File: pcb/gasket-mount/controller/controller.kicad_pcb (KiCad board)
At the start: 2 copper layers, 31.3 x 24.9 mm, 34 parts, among them J1 USB_C_Receptacle_USB2.0_16P, U1 USBLC6-2SC6, U3 W25Q128JVP, U4 RP2040, U5 AP2112K-3.3, X1 ABM8-272-T3

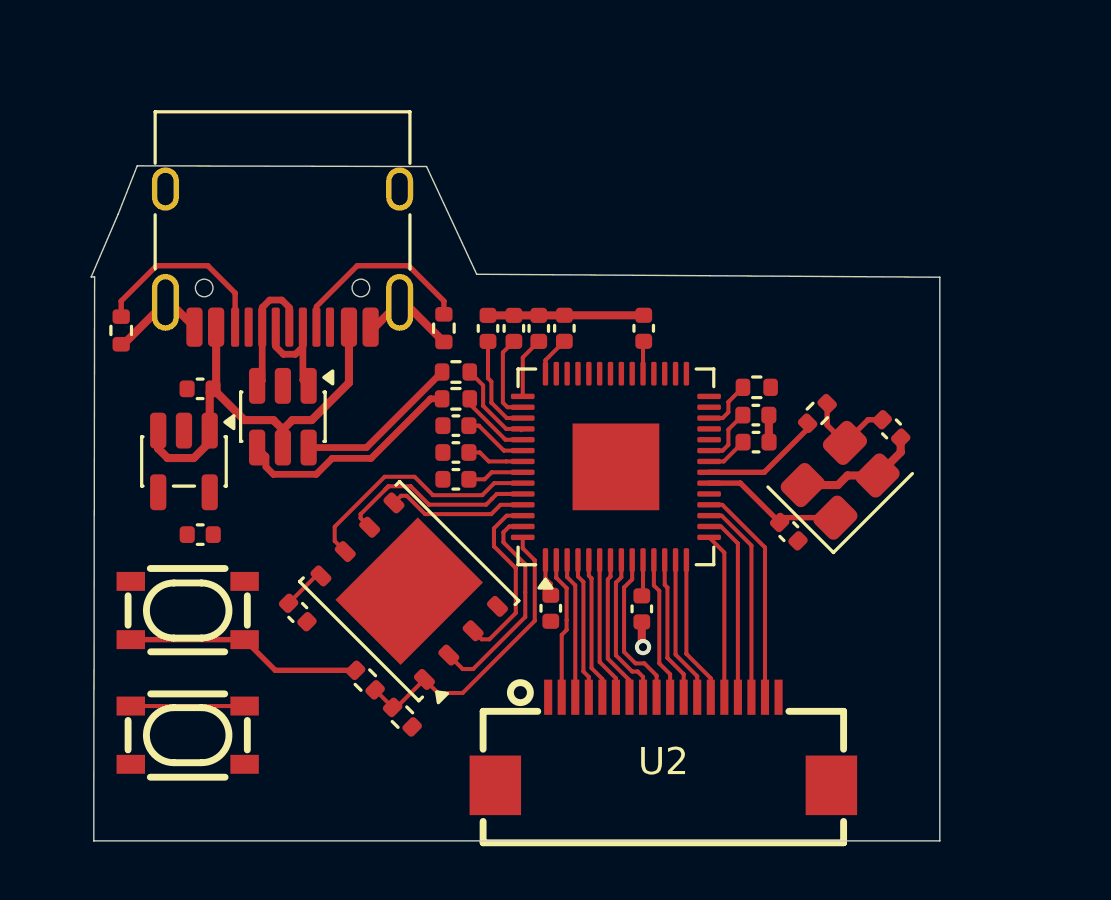
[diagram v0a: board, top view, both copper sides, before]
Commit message: Last commit before changing Flash memory
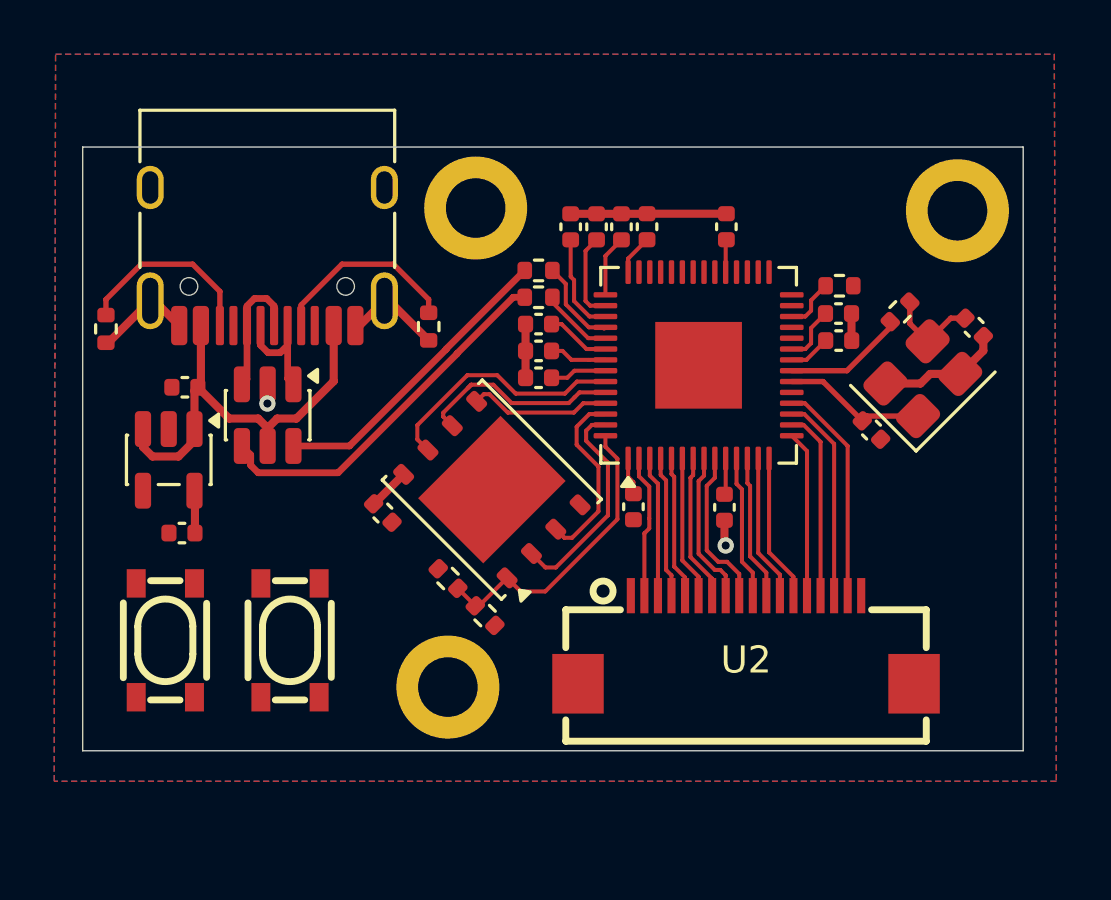
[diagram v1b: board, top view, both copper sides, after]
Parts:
- added H1: MountingHole_Pad, MountingHole:MountingHole_2.2mm_M2_ISO14580_Pad, F.Cu at (83.0, 78.8)
- added H2: MountingHole_Pad, MountingHole:MountingHole_2.2mm_M2_ISO14580_Pad, F.Cu at (84.0, 61.1)
- added H3: MountingHole_Pad, MountingHole:MountingHole_2.2mm_M2_ISO14580_Pad, F.Cu at (101.8, 61.2)
- moved SW3 5.15 mm to (77.2, 77.1), turned to -90 degrees
- moved C16 4.83 mm to (86.3, 66.4)
- moved C5 4.83 mm to (102.4, 65.6)
- moved R5 4.83 mm to (99.7, 65.0)
- moved C17 4.83 mm to (86.3, 65.4)
- moved C6 4.83 mm to (97.4, 66.0)
- moved R3 4.83 mm to (84.4, 76.2)
- moved U2 4.83 mm to (94.0, 77.1)
- moved U4 4.83 mm to (92.2, 67.0)
- moved C4 4.83 mm to (98.6, 69.3)
- moved R8 4.83 mm to (86.3, 64.4)
- moved X1 4.83 mm to (100.5, 67.4)
- moved C14 4.83 mm to (89.4, 61.8)
- moved C15 4.83 mm to (90.3, 61.8)
- moved C7 4.83 mm to (93.3, 61.8)
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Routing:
- net /BOOT: track 8.76 -> 0.00 mm
- net DATA+: track 8.61 -> 13.8 mm
- net DATA-: track 6.08 -> 11.2 mm
- net /RESET: track 6.14 -> 1.94 mm
- net GND: track 19.7 -> 22.4 mm, vias 1 -> 2
- net +3V3: track 18.6 -> 20.3 mm
- added copper zone on B.Cu, net GND
- added copper zone on F.Cu, net GND
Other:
- board size 31.3 x 24.9 mm -> 34.7 x 22.3 mm
